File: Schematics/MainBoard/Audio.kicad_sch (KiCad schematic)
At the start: 20 parts, among them J6 AudioJack3, U11 LM386, U16 MCP6022

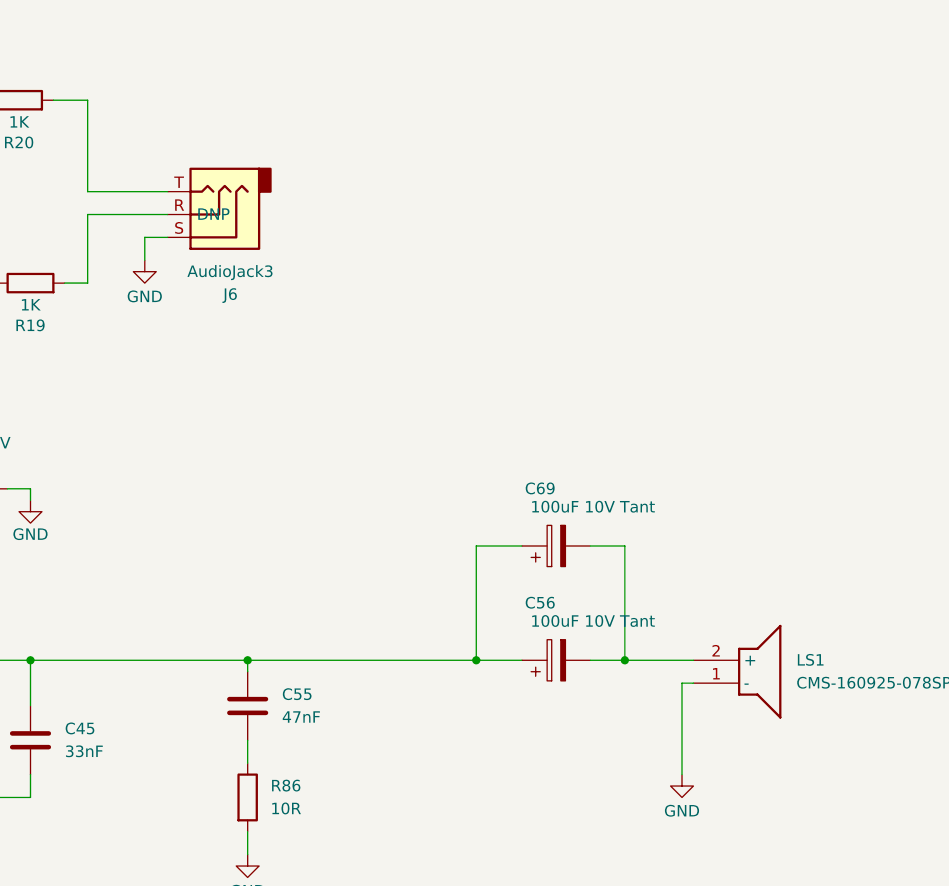
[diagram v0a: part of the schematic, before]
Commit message: Updates based on production files for JLC
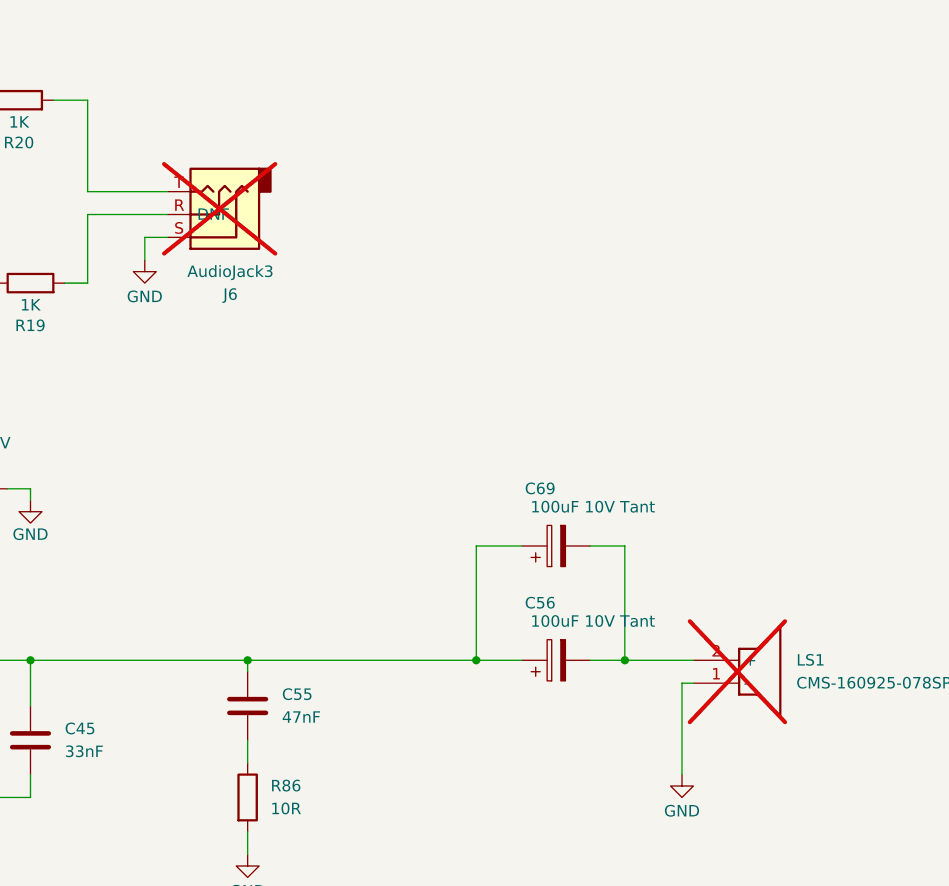
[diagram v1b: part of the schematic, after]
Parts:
- C43: LCSC (none) -> C21120
- C44, C46: LCSC C113803 -> C307331
- C55: LCSC C1622 -> C82219
- C56, C69: LCSC DNP -> C49332976
- J6: LCSC DNP -> DNF; now not fitted
- LS1: now not fitted
- R19, R20: LCSC (none) -> C11702
- R23, R88: LCSC DNF -> C25792
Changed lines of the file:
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@@
 		(in_bom yes)
 		(on_board yes)
-		(dnp no)
+		(dnp yes)
 		(property "Reference" "J6"
 			(at 186.055 52.07 0)
@@
 			)
 		)
-		(property "LCSC" "DNP"
+		(property "LCSC" "DNF"
 			(at 184.15 43.18 0)
 			(effects
@@
 			)
 		)
-		(property "LCSC" "DNF"
+		(property "LCSC" "C25792"
 			(at 58.42 154.94 90)
 			(effects
@@
 			)
 		)
-		(property "LCSC" ""
+		(property "LCSC" "C11702"
 			(at 163.83 50.8 90)
 			(effects
@@
 			)
 		)
-		(property "LCSC" "DNP"
+		(property "LCSC" "C49332976"
 			(at 222.25 80.01 0)
 			(effects
@@
 			)
 		)
-		(property "LCSC" ""
+		(property "LCSC" "C21120"
 			(at 110.49 40.64 0)
 			(effects
@@
 			)
 		)
-		(property "LCSC" "C113803"
+		(property "LCSC" "C307331"
 			(at 45.72 27.94 0)
 			(effects
@@
 			)
 		)
-		(property "LCSC" ""
+		(property "LCSC" "C11702"
 			(at 162.56 30.48 90)
 			(effects
@@
 		(in_bom yes)
 		(on_board yes)
-		(dnp no)
+		(dnp yes)
 		(fields_autoplaced yes)
 		(property "Reference" "LS1"
@@
 			)
 		)
-		(property "LCSC" "DNF"
+		(property "LCSC" "C25792"
 			(at 66.04 133.35 90)
 			(effects
@@
 			)
 		)
-		(property "LCSC" "C113803"
+		(property "LCSC" "C307331"
 			(at 124.46 80.01 0)
 			(effects
@@
 			)
 		)
-		(property "LCSC" "DNP"
+		(property "LCSC" "C49332976"
 			(at 222.25 92.71 0)
 			(effects
@@
 			)
 		)
-		(property "LCSC" "C1622"
+		(property "LCSC" "C82219"
 			(at 187.96 97.79 0)
 			(effects
